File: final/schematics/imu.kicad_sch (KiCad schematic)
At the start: 10 parts, among them U1 BMI270, U2 BMI270

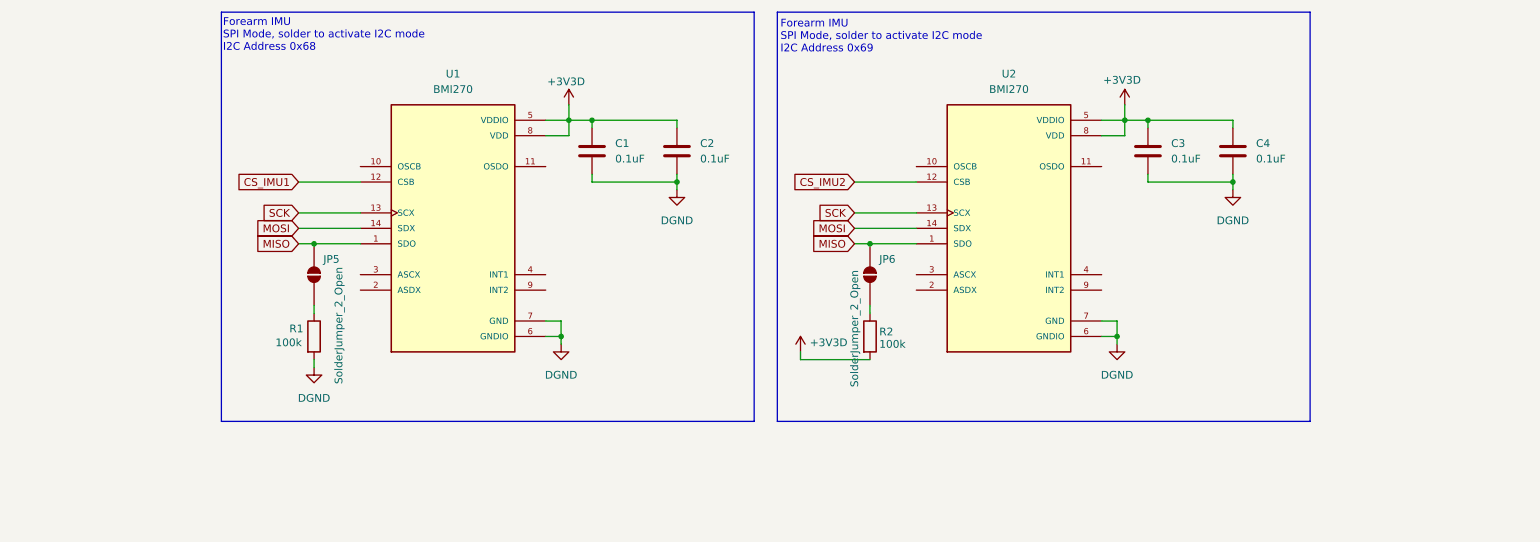
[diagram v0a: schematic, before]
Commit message: fixing
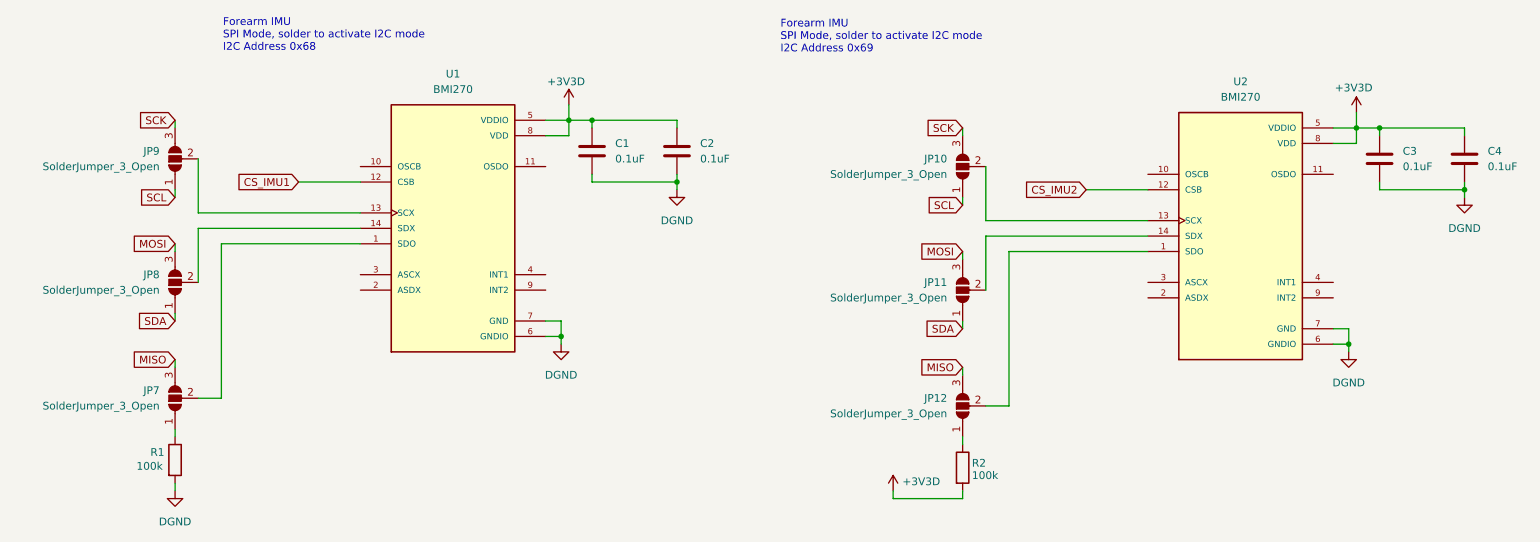
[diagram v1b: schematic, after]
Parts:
- removed JP5, JP6: SolderJumper_2_Open, Jumper:SolderJumper-2_P1.3mm_Open_RoundedPad1.0x1.5mm, symbol Jumper:SolderJumper_2_Open
- added JP10, JP11, JP12, JP7, JP8, JP9: SolderJumper_3_Open, Jumper:SolderJumper-3_P1.3mm_Open_RoundedPad1.0x1.5mm, symbol Jumper:SolderJumper_3_Open
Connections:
- net MISO: now also JP12.3 (B), JP7.3 (B); no longer U1.1 (SDO), U2.1 (SDO)
- net MOSI: now also JP11.3 (B), JP8.3 (B); no longer U1.14 (SDX), U2.14 (SDX)
- net SCK: now also JP10.3 (B), JP9.3 (B); no longer U1.13 (SCX), U2.13 (SCX)
- net at R2.1: now also JP12.1 (A)
- net at R1.1: now also JP7.1 (A)
- new net: JP8.2 (C), U1.14 (SDX)
- new net: JP10.2 (C), U2.13 (SCX)
- new net: JP12.2 (C), U2.1 (SDO)
- new net: JP9.2 (C), U1.13 (SCX)
- new net: JP7.2 (C), U1.1 (SDO)
- new net: JP11.2 (C), U2.14 (SDX)
- new net SCL: JP10.1 (A), JP9.1 (A)
- new net SDA: JP11.1 (A), JP8.1 (A)
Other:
- moved on the sheet: C3, C4, R1, R2, U2
